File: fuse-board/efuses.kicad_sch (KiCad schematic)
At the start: 42 parts, among them U4 PTPS259830LNRGER, U5 PTPS259830LNRGER, U6 PTPS259830LNRGER, U7 PTPS259830LNRGER, U8 PTPS259830LNRGER, U9 PTPS259830LNRGER

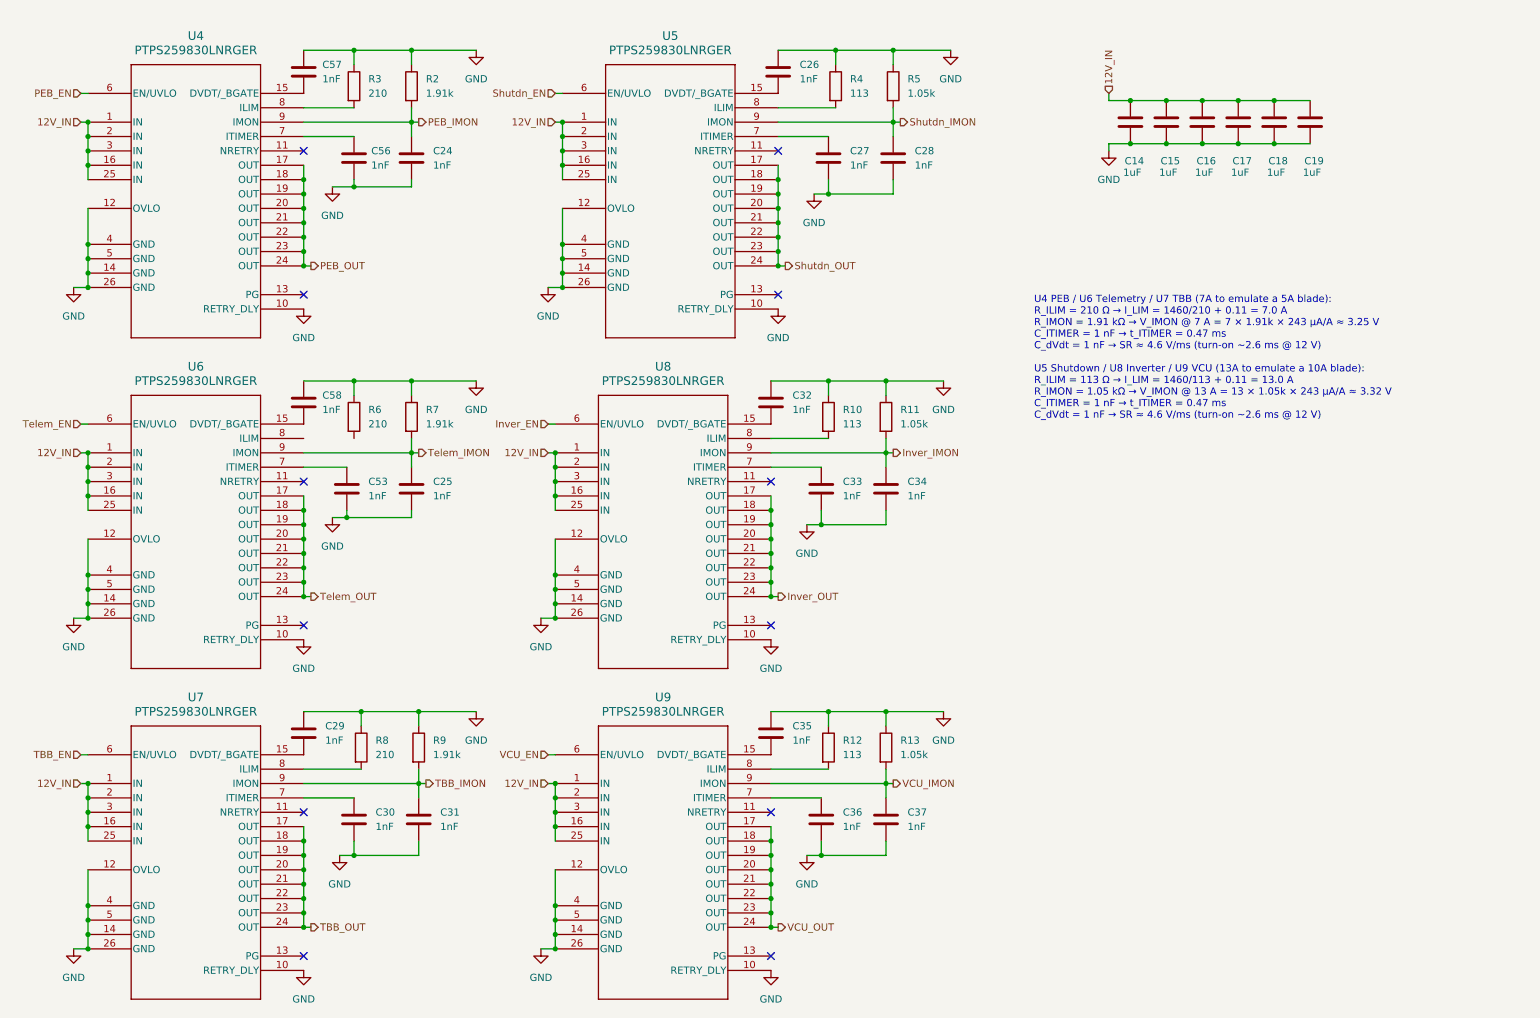
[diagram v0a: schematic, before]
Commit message: switch efuse config and symbol
passives still need to be sourced
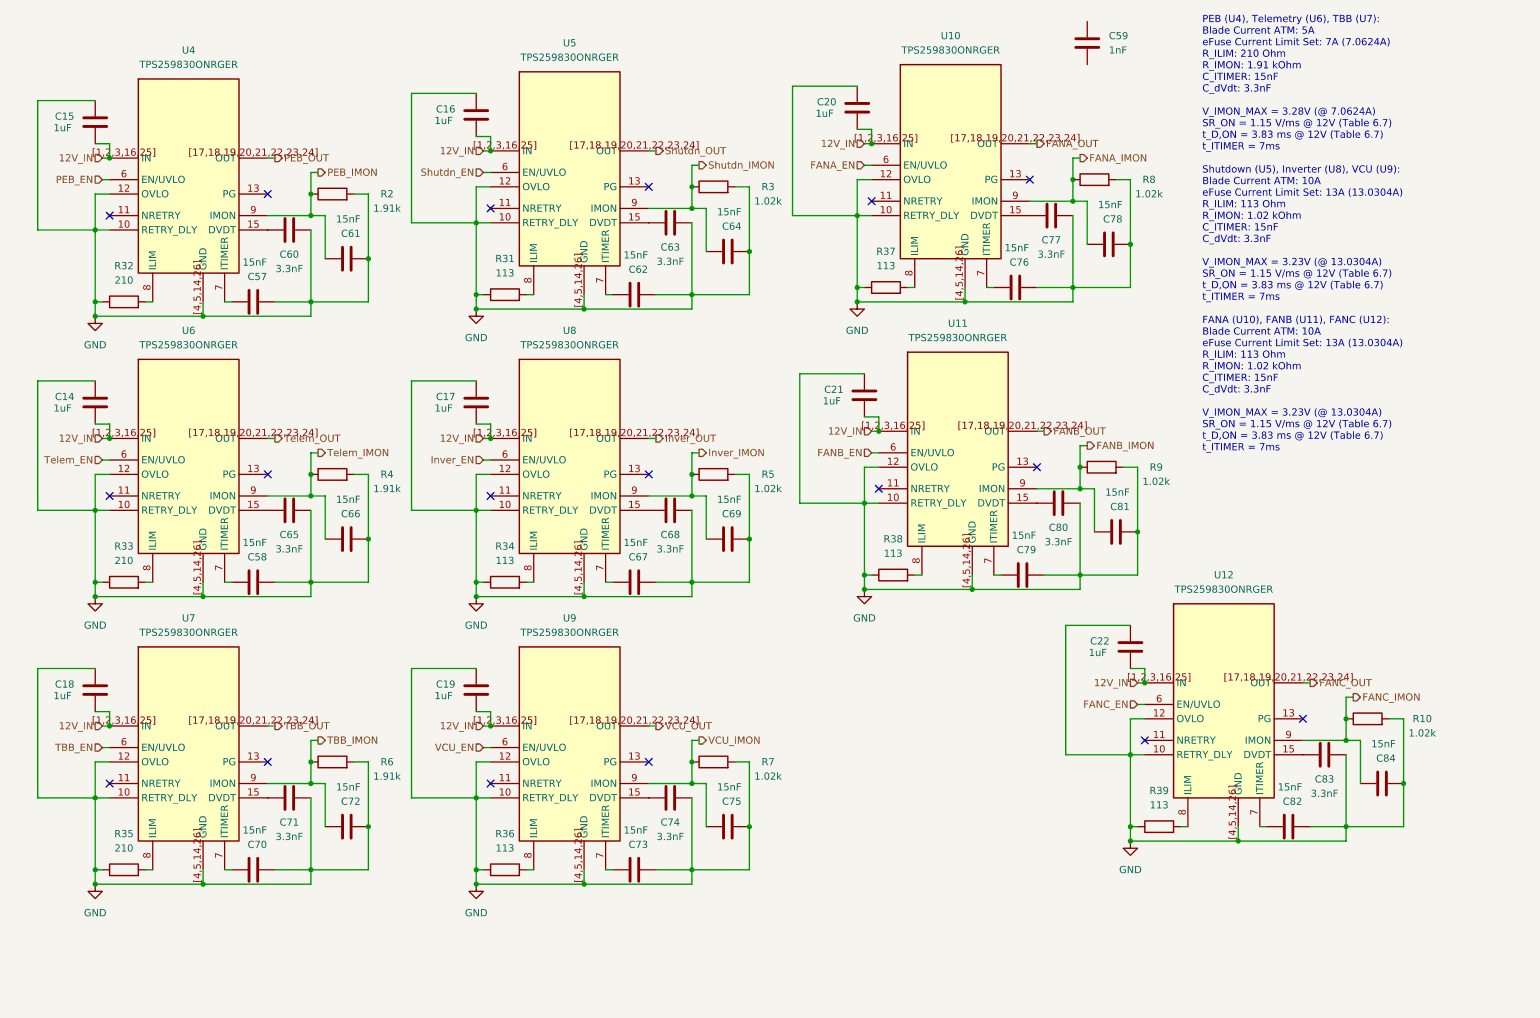
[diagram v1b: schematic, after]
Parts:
- removed C24, C25, C26, C27, C28, C29, C30, C31, C32, C33, C34, C35, C36, C37, C53, C56: 1nF, Capacitor_SMD:C_0603_1608Metric_Pad1.08x0.95mm_HandSolder, symbol Device:C
- removed R11, R13: 1.05k, Resistor_SMD:R_0603_1608Metric_Pad0.98x0.95mm_HandSolder, symbol Device:R
- removed R12: 113, Resistor_SMD:R_0603_1608Metric_Pad0.98x0.95mm_HandSolder, symbol Device:R
- removed U4, U5, U6, U7, U8, U9: PTPS259830LNRGER, formula_slug_footprint_library:VQFN24_RGE_TEX, symbol formula_slug_symbol_library:PTPS259830LNRGER
- added C20, C21, C22: 1uF, Capacitor_SMD:C_0603_1608Metric_Pad1.08x0.95mm_HandSolder, symbol Device:C
- added C59: 1nF, Capacitor_SMD:C_0603_1608Metric_Pad1.08x0.95mm_HandSolder, symbol Device:C
- added C60, C63, C65, C68, C71, C74, C77, C80, C83: 3.3nF, Capacitor_SMD:C_0603_1608Metric_Pad1.08x0.95mm_HandSolder, symbol Device:C
- added C61, C62, C64, C66, C67, C69, C70, C72, C73, C75, C76, C78, C79, C81, C82, C84: 15nF, Capacitor_SMD:C_0603_1608Metric_Pad1.08x0.95mm_HandSolder, symbol Device:C
- added R31, R34, R36, R37, R38, R39: 113, Resistor_SMD:R_0603_1608Metric_Pad0.98x0.95mm_HandSolder, symbol Device:R
- added R32, R33, R35: 210, Resistor_SMD:R_0603_1608Metric_Pad0.98x0.95mm_HandSolder, symbol Device:R
- added U10, U11, U12, U4, U5, U6, U7, U8, U9: TPS259830ONRGER, formula_slug_footprint_library:TPS259830ONRGER, symbol formula_slug_symbol_library:TPS259830ONRGER
- C57, C58: value 1nF -> 15nF; Digikey Part Number 311-1423-1-ND -> (none); Digikey URL https://www.digikey.com/en/products/detail/yageo/CC0603JRNP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 -> (none); Manufacturer YAGEO -> (none); Manufacturer Part Number CC0603JRNPO9BN102 -> (none)
- R10: value 113 -> 1.02k; Digikey Part Number 311-113HRCT-ND -> (none); Digikey URL https://www.digikey.com/en/products/detail/yageo/RC0603FR-0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 -> (none); Manufacturer YAGEO -> (none); Manufacturer Part Number RC0603FR-07113RL -> (none)
- R3, R8: value 210 -> 1.02k; Digikey Part Number 311-210HRCT-ND -> (none); Digikey URL https://www.digikey.com/en/products/detail/yageo/RC0603FR-0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 -> (none); Manufacturer YAGEO -> (none); Manufacturer Part Number RC0603FR-07210RL -> (none)
- R4: value 113 -> 1.91k; Digikey Part Number 311-113HRCT-ND -> 13-AC0603FR-071K91LCT-ND; Digikey URL https://www.digikey.com/en/products/detail/yageo/RC0603FR-0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 -> https://www.digikey.com/en/products/detail/yageo/AC0603FR-0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; Manufacturer Part Number RC0603FR-07113RL -> AC0603FR-071K91L
- R5: value 1.05k -> 1.02k; Digikey Part Number 311-1.05KHRCT-ND -> (none); Digikey URL https://www.digikey.com/en/products/detail/yageo/RC0603FR-0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 -> (none); Manufacturer YAGEO -> (none); Manufacturer Part Number RC0603FR-071K05L -> (none)
- R6: value 210 -> 1.91k; Digikey Part Number 311-210HRCT-ND -> 13-AC0603FR-071K91LCT-ND; Digikey URL https://www.digikey.com/en/products/detail/yageo/RC0603FR-0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 -> https://www.digikey.com/en/products/detail/yageo/AC0603FR-0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; Manufacturer Part Number RC0603FR-07210RL -> AC0603FR-071K91L
- R7, R9: value 1.91k -> 1.02k; Digikey Part Number 13-AC0603FR-071K91LCT-ND -> (none); Digikey URL https://www.digikey.com/en/products/detail/yageo/AC0603FR-0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 -> (none); Manufacturer YAGEO -> (none); Manufacturer Part Number AC0603FR-071K91L -> (none)
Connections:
- net 12V_IN: now also C14.2, C15.2, C16.2, C17.2, C18.2, C19.2, C20.2, C21.2, C22.2, U10.[1,2,3,16,25] (IN), U11.[1,2,3,16,25] (IN), U12.[1,2,3,16,25] (IN), U4.[1,2,3,16,25] (IN), U5.[1,2,3,16,25] (IN), U6.[1,2,3,16,25] (IN), U7.[1,2,3,16,25] (IN), U8.[1,2,3,16,25] (IN), U9.[1,2,3,16,25] (IN); no longer C14.1, C15.1, C16.1, C17.1, C18.1, C19.1
- net GND: now also C14.1, C15.1, C16.1, C17.1, C18.1, C19.1, C57.2, C58.2, R10.2, R2.2, R3.2, R4.2, R5.2, R6.2, R7.2, R8.2, R9.2, C20.1, C21.1, C22.1, C60.2, C61.2, C62.2, C63.2, C64.2, C65.2, C66.2, C67.2, C68.2, C69.2, C70.2, C71.2, C72.2, C73.2, C74.2, C75.2, C76.2, C77.2, C78.2, C79.2, C80.2, C81.2, C82.2, C83.2, C84.2, R31.1, R32.1, R33.1, R34.1, R35.1, R36.1, R37.1, R38.1, R39.1, U10.10 (RETRY_DLY), U10.12 (OVLO), U10.[4,5,14,26] (GND), U11.10 (RETRY_DLY), U11.12 (OVLO), U11.[4,5,14,26] (GND), U12.10 (RETRY_DLY), U12.12 (OVLO), U12.[4,5,14,26] (GND), U4.10 (RETRY_DLY), U4.12 (OVLO), U4.[4,5,14,26] (GND), U5.10 (RETRY_DLY), U5.12 (OVLO), U5.[4,5,14,26] (GND), U6.10 (RETRY_DLY), U6.12 (OVLO), U6.[4,5,14,26] (GND), U7.10 (RETRY_DLY), U7.12 (OVLO), U7.[4,5,14,26] (GND), U8.10 (RETRY_DLY), U8.12 (OVLO), U8.[4,5,14,26] (GND), U9.10 (RETRY_DLY), U9.12 (OVLO), U9.[4,5,14,26] (GND); no longer C14.2, C15.2, C16.2, C17.2, C18.2, C19.2, C57.1, C58.1, R10.1, R2.1, R3.1, R4.1, R5.1, R6.1, R7.1, R8.1, R9.1
- net Inver_EN: now also U8.6 (EN/UVLO)
- net Inver_IMON: now also R5.1, C69.1, U8.9 (IMON)
- net Inver_OUT: now also U8.[17,18,19,20,21,22,23,24] (OUT)
- net PEB_EN: now also U4.6 (EN/UVLO)
- net PEB_IMON: now also R2.1, C61.1, U4.9 (IMON); no longer R2.2
- net PEB_OUT: now also U4.[17,18,19,20,21,22,23,24] (OUT)
- net Shutdn_EN: now also U5.6 (EN/UVLO)
- net Shutdn_IMON: now also R3.1, C64.1, U5.9 (IMON); no longer R5.2
- net Shutdn_OUT: now also U5.[17,18,19,20,21,22,23,24] (OUT)
- net TBB_EN: now also U7.6 (EN/UVLO)
- net TBB_IMON: now also R6.1, C72.1, U7.9 (IMON); no longer R9.2
- net TBB_OUT: now also U7.[17,18,19,20,21,22,23,24] (OUT)
- net Telem_EN: now also U6.6 (EN/UVLO)
- net Telem_IMON: now also R4.1, C66.1, U6.9 (IMON); no longer R7.2
- net Telem_OUT: now also U6.[17,18,19,20,21,22,23,24] (OUT)
- net VCU_EN: now also U9.6 (EN/UVLO)
- net VCU_IMON: now also R7.1, C75.1, U9.9 (IMON)
- net VCU_OUT: now also U9.[17,18,19,20,21,22,23,24] (OUT)
- new net: C60.1, U4.15 (DVDT)
- new net: C57.1, U4.7 (ITIMER)
- new net: R32.2, U4.8 (ILIM)
- new net: R38.2, U11.8 (ILIM)
- new net: C63.1, U5.15 (DVDT)
- new net: C62.1, U5.7 (ITIMER)
- new net: R31.2, U5.8 (ILIM)
- new net: R33.2, U6.8 (ILIM)
- new net: C74.1, U9.15 (DVDT)
- new net: C73.1, U9.7 (ITIMER)
- new net: R36.2, U9.8 (ILIM)
- new net: C71.1, U7.15 (DVDT)
- new net: R37.2, U10.8 (ILIM)
- new net: C70.1, U7.7 (ITIMER)
- new net: R35.2, U7.8 (ILIM)
- new net: C65.1, U6.15 (DVDT)
- new net: C80.1, U11.15 (DVDT)
- new net: C79.1, U11.7 (ITIMER)
- new net: C83.1, U12.15 (DVDT)
- new net: C68.1, U8.15 (DVDT)
- new net: C67.1, U8.7 (ITIMER)
- new net: R34.2, U8.8 (ILIM)
- new net: C58.1, U6.7 (ITIMER)
- new net: C82.1, U12.7 (ITIMER)
- new net: R39.2, U12.8 (ILIM)
- new net: C77.1, U10.15 (DVDT)
- new net: C76.1, U10.7 (ITIMER)
- new net FANA_EN: U10.6 (EN/UVLO)
- new net FANA_IMON: C78.1, R8.1, U10.9 (IMON)
- new net FANA_OUT: U10.[17,18,19,20,21,22,23,24] (OUT)
- new net FANB_EN: U11.6 (EN/UVLO)
- new net FANB_IMON: C81.1, R9.1, U11.9 (IMON)
- new net FANB_OUT: U11.[17,18,19,20,21,22,23,24] (OUT)
- new net FANC_EN: U12.6 (EN/UVLO)
- new net FANC_IMON: C84.1, R10.1, U12.9 (IMON)
- new net FANC_OUT: U12.[17,18,19,20,21,22,23,24] (OUT)
- no-connect marks 12 -> 18
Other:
- note added: "PEB (U4), Telemetry (U6), TBB (U7): Blade Current ATM: 5A eFuse Current Limit Set: 7A (7.0624A) R_ILIM: 210 Ohm R_IMON: 1.91 kOhm C_ITIMER: 15nF C_dVdt: 3.3nF V_IMON_MAX = 3.28V (@ 7.0624A) SR_ON = 1.15 V/ms @ 12V (Table 6.7) t_D,ON = 3.83 ms @ 12V (Table 6.7) t_ITIMER = 7ms Shutdown (U5), Inverter (U8), VCU (U9): Blade Current ATM: 10A eFuse Current Limit Set: 13A (13.0304A) R_ILIM: 113 Ohm R_IM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"
- note removed: "U4 PEB / U6 Telemetry / U7 TBB (7A to emulate a 5A blade): R_ILIM = 210 Ω → I_LIM = 1460/210 + 0.11 = 7.0 A R_IMON = 1.91 kΩ → V_IMON @ 7 A = 7 × 1.91k × 243 µA/A ≈ 3.25 V C_ITIMER = 1 nF → t_ITIMER = 0.47 ms C_dVdt = 1 nF → SR ≈ 4.6 V/ms (turn-on ~2.6 ms @ 12 V) U5 Shutdown / U8 Inverter / U9 VCU (13A to emulate a 10A blade): R_ILIM = 113 Ω → I_LIM = 1460/113 + 0.11 = 13.0 A R_IMON = 1.05 kΩ → V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"
- moved on the sheet: C14, C57, R2
